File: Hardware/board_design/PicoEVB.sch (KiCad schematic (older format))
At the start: 0 parts

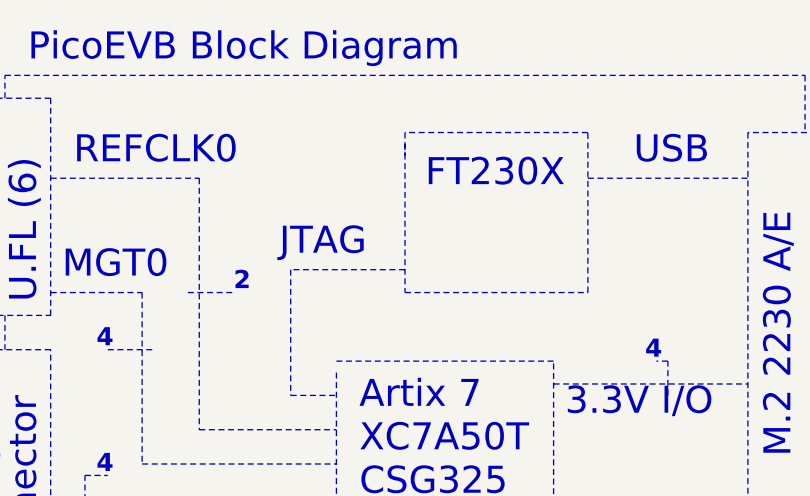
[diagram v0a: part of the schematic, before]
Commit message: rescured and remaped symbols
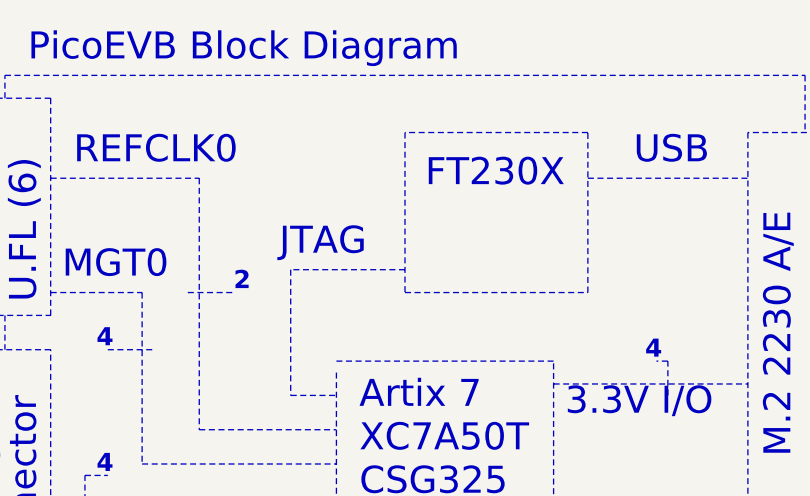
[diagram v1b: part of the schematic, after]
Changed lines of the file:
@@
-EESchema Schematic File Version 2
-LIBS:power
-LIBS:device
-LIBS:transistors
-LIBS:conn
-LIBS:linear
-LIBS:regul
-LIBS:74xx
-LIBS:cmos4000
-LIBS:adc-dac
-LIBS:memory
-LIBS:xilinx
-LIBS:microcontrollers
-LIBS:dsp
-LIBS:microchip
-LIBS:analog_switches
-LIBS:motorola
-LIBS:texas
-LIBS:intel
-LIBS:audio
-LIBS:interface
-LIBS:digital-audio
-LIBS:philips
-LIBS:display
-LIBS:cypress
-LIBS:siliconi
-LIBS:opto
-LIBS:atmel
-LIBS:contrib
-LIBS:valves
-LIBS:Zilog
-LIBS:zetex
-LIBS:Xicor
-LIBS:Worldsemi
-LIBS:wiznet
-LIBS:video
-LIBS:ttl_ieee
-LIBS:transf
-LIBS:switches
-LIBS:supertex
-LIBS:stm32
-LIBS:stm8
-LIBS:silabs
-LIBS:sensors
-LIBS:rfcom
-LIBS:relays
-LIBS:references
-LIBS:pspice
-LIBS:Power_Management
-LIBS:powerint
-LIBS:Oscillators
-LIBS:onsemi
-LIBS:nxp_armmcu
-LIBS:nordicsemi
-LIBS:msp430
-LIBS:motors
-LIBS:motor_drivers
-LIBS:microchip_pic32mcu
-LIBS:microchip_pic18mcu
-LIBS:microchip_pic16mcu
-LIBS:microchip_pic12mcu
-LIBS:microchip_pic10mcu
-LIBS:microchip_dspic33dsc
-LIBS:mechanical
-LIBS:maxim
-LIBS:logo
-LIBS:Lattice
-LIBS:ir
-LIBS:hc11
-LIBS:graphic
-LIBS:gennum
-LIBS:ftdi
-LIBS:ESD_Protection
-LIBS:elec-unifil
-LIBS:diode
-LIBS:dc-dc
-LIBS:cmos_ieee
-LIBS:brooktre
-LIBS:bosch
-LIBS:bbd
-LIBS:battery_management
-LIBS:analog_devices
-LIBS:Altera
-LIBS:allegro
-LIBS:actel
-LIBS:ac-dc
-LIBS:74xgxx
-LIBS:xc7a50t-bga325
-LIBS:MAX1589A
-LIBS:MIC47050
-LIBS:TS3L110
-LIBS:W25Q
-LIBS:93LC46B-SOT23
-LIBS:m2-board
-LIBS:ft2232-fixed
-LIBS:tps82084
-LIBS:PicoEVB-cache
-EELAYER 25 0
+EESchema Schematic File Version 4
+EELAYER 30 0
 EELAYER END
 $Descr A 11000 8500
@@
 	6950 2000 6650 2000
 Wire Notes Line
-	5150 2050 5150 2700
-Wire Notes Line
 	5150 2700 5950 2700
 Wire Notes Line
@@
 Wire Notes Line
 	5950 2000 5150 2000
-Wire Notes Line
-	5150 2000 5150 2100
 Text Notes 5850 2250 2    118  ~ 0
 FT230X
@@
 Wire Notes Line
 	6300 3900 6300 4000
+Wire Notes Line
+	5150 2000 5150 2700
 $EndSCHEMATC
